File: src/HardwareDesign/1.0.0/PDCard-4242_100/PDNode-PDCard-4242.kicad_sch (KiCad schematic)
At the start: 0 parts

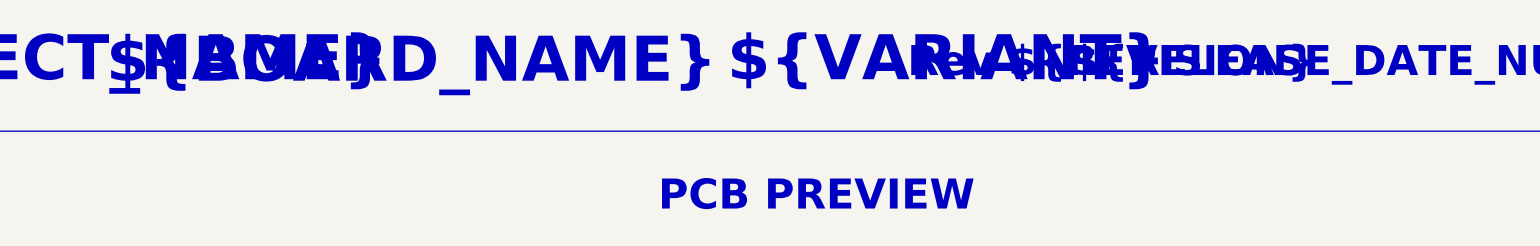
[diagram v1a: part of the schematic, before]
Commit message: update readme, add documentation
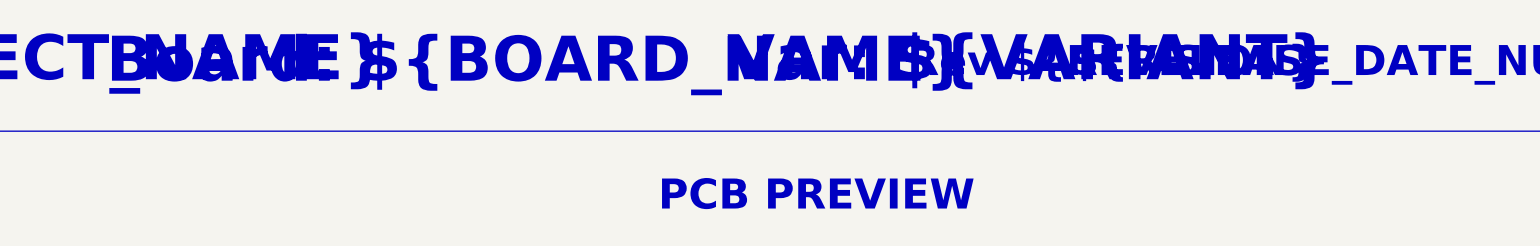
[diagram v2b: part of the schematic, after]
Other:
- note added: "Board: ${BOARD_NAME}"
- note added: "Var: ${VARIANT}"
- note removed: "${BOARD_NAME}"
- note removed: "${VARIANT}"
